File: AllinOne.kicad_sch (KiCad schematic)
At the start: 268 parts, among them SW0 SW_Push, SW1 SW_Push, SW10 SW_Push, SW100 SW_Push, SW101 SW_Push, SW102 SW_Push, SW103 SW_Push, SW104 SW_Push, SW105 SW_Push, SW106 SW_Push, SW107 SW_Push, SW108 SW_Push, SW109 SW_Push, SW11 SW_Push, SW110 SW_Push, SW111 SW_Push, SW114 SW_Push, SW116 SW_Push, SW117 SW_Push, SW118 SW_Push, SW119 SW_Push, SW12 SW_Push, SW120 SW_Push, SW121 SW_Push, SW122 SW_Push, SW126 SW_Push, SW13 SW_Push, SW130 SW_Push, SW131 SW_Push, SW132 SW_Push, SW133 SW_Push, SW134 SW_Push, SW135 SW_Push, SW136 SW_Push, SW137 SW_Push, SW138 SW_Push, SW139 SW_Push, SW14 SW_Push, SW15 SW_Push, SW16 SW_Push, SW18 SW_Push, SW19 SW_Push, SW2 SW_Push, SW20 SW_Push, SW21 SW_Push, SW22 SW_Push, SW23 SW_Push, SW24 SW_Push, SW25 SW_Push, SW26 SW_Push, SW27 SW_Push, SW28 SW_Push, SW29 SW_Push, SW3 SW_Push, SW30 SW_Push, SW31 SW_Push, SW32 SW_Push, SW33 SW_Push, SW34 SW_Push, SW35 SW_Push, SW36 SW_Push, SW37 SW_Push, SW38 SW_Push, SW39 SW_Push, SW4 SW_Push, SW40 SW_Push, SW41 SW_Push, SW42 SW_Push, SW43 SW_Push, SW44 SW_Push, SW45 SW_Push, SW46 SW_Push, SW47 SW_Push, SW48 SW_Push, SW49 SW_Push, SW5 SW_Push, SW50 SW_Push, SW51 SW_Push, SW52 SW_Push, SW53 SW_Push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

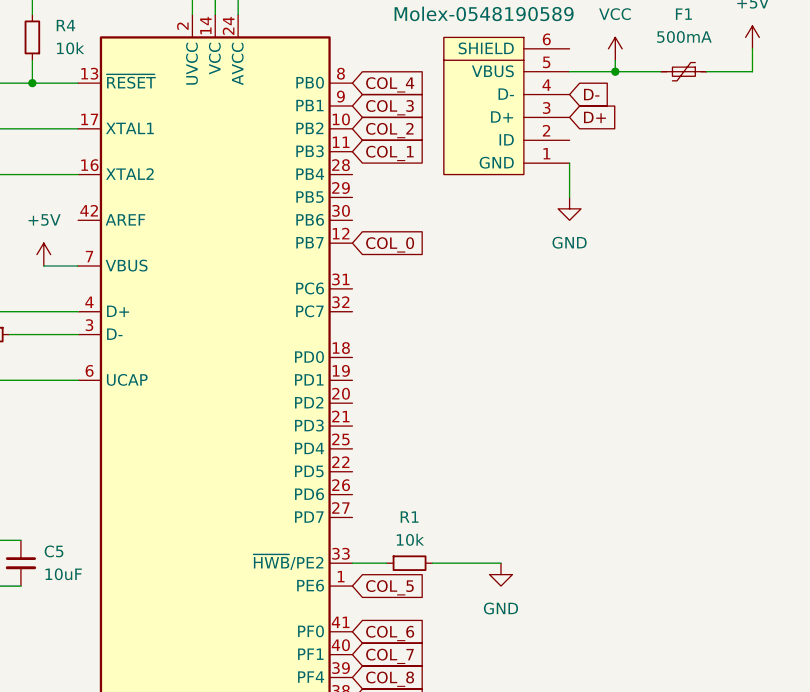
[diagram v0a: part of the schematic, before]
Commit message: All Done for now
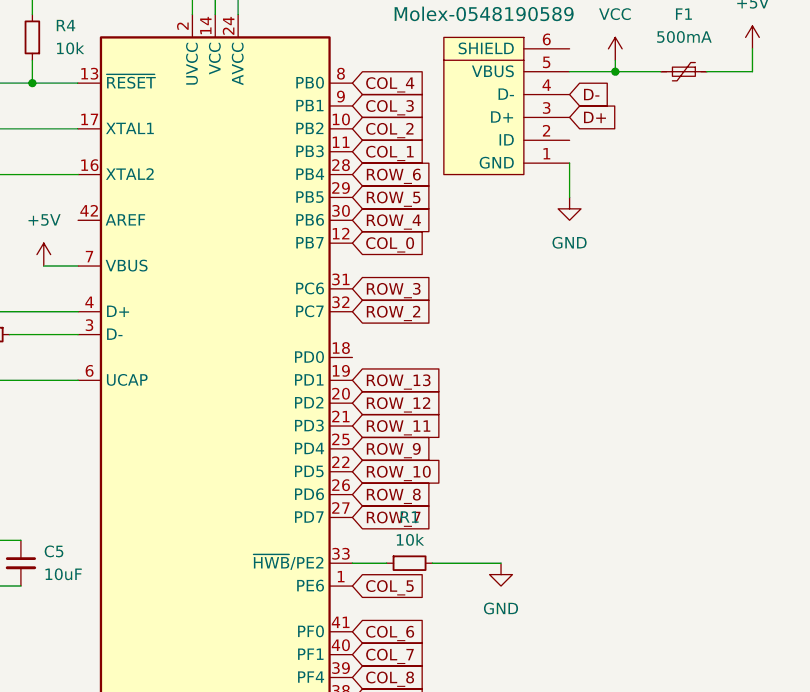
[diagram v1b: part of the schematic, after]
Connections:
- net ROW_10: now also U1.22 (PD5)
- net ROW_11: now also U1.21 (PD3)
- net ROW_12: now also U1.20 (PD2)
- net ROW_13: now also U1.19 (PD1)
- net ROW_2: now also U1.32 (PC7)
- net ROW_3: now also U1.31 (PC6)
- net ROW_4: now also U1.30 (PB6)
- net ROW_5: now also U1.29 (PB5)
- net ROW_6: now also U1.28 (PB4)
- net ROW_7: now also U1.27 (PD7)
- net ROW_8: now also U1.26 (PD6)
- net ROW_9: now also U1.25 (PD4)
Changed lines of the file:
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@@
     (stroke (width 0) (type default))
   )
+  (global_label "ROW_5" (shape input) (at 87.63 191.77 0) (fields_autoplaced)
+    (effects (font (size 1.27 1.27)) (justify left))
+    (property "Intersheetrefs" "${INTERSHEET_REFS}" (at 96.7648 191.77 0)
+      (effects (font (size 1.27 1.27)) (justify left) hide)
+    )
+  )
   (global_label "COL_6" (shape input) (at 289.56 27.94 90) (fields_autoplaced)
     (effects (font (size 1.27 1.27)) (justify left))
@@
     )
   )
+  (global_label "ROW_6" (shape input) (at 87.63 189.23 0) (fields_autoplaced)
+    (effects (font (size 1.27 1.27)) (justify left))
+    (property "Intersheetrefs" "${INTERSHEET_REFS}" (at 96.7648 189.23 0)
+      (effects (font (size 1.27 1.27)) (justify left) hide)
+    )
+  )
+  (global_label "ROW_10" (shape input) (at 87.63 222.25 0) (fields_autoplaced)
+    (effects (font (size 1.27 1.27)) (justify left))
+    (property "Intersheetrefs" "${INTERSHEET_REFS}" (at 97.9743 222.25 0)
+      (effects (font (size 1.27 1.27)) (justify left) hide)
+    )
+  )
   (global_label "ROW_7" (shape input) (at 30.48 109.22 180) (fields_autoplaced)
     (effects (font (size 1.27 1.27)) (justify right))
@@
     )
   )
+  (global_label "ROW_2" (shape input) (at 87.63 204.47 0) (fields_autoplaced)
+    (effects (font (size 1.27 1.27)) (justify left))
+    (property "Intersheetrefs" "${INTERSHEET_REFS}" (at 96.7648 204.47 0)
+      (effects (font (size 1.27 1.27)) (justify left) hide)
+    )
+  )
   (global_label "COL_0" (shape input) (at 76.2 27.94 90) (fields_autoplaced)
     (effects (font (size 1.27 1.27)) (justify left))
@@
     )
   )
+  (global_label "ROW_7" (shape input) (at 87.63 227.33 0) (fields_autoplaced)
+    (effects (font (size 1.27 1.27)) (justify left))
+    (property "Intersheetrefs" "${INTERSHEET_REFS}" (at 96.7648 227.33 0)
+      (effects (font (size 1.27 1.27)) (justify left) hide)
+    )
+  )
   (global_label "COL_7" (shape input) (at 87.63 242.57 0) (fields_autoplaced)
     (effects (font (size 1.27 1.27)) (justify left))
@@
     )
   )
+  (global_label "ROW_8" (shape input) (at 87.63 224.79 0) (fields_autoplaced)
+    (effects (font (size 1.27 1.27)) (justify left))
+    (property "Intersheetrefs" "${INTERSHEET_REFS}" (at 96.7648 224.79 0)
+      (effects (font (size 1.27 1.27)) (justify left) hide)
+    )
+  )
   (global_label "ROW_0" (shape input) (at 87.63 250.19 0) (fields_autoplaced)
     (effects (font (size 1.27 1.27)) (justify left))
@@
     )
   )
+  (global_label "ROW_12" (shape input) (at 87.63 214.63 0) (fields_autoplaced)
+    (effects (font (size 1.27 1.27)) (justify left))
+    (property "Intersheetrefs" "${INTERSHEET_REFS}" (at 97.9743 214.63 0)
+      (effects (font (size 1.27 1.27)) (justify left) hide)
+    )
+  )
   (global_label "COL_3" (shape input) (at 182.88 27.94 90) (fields_autoplaced)
     (effects (font (size 1.27 1.27)) (justify left))
@@
     )
   )
+  (global_label "ROW_3" (shape input) (at 87.63 201.93 0) (fields_autoplaced)
+    (effects (font (size 1.27 1.27)) (justify left))
+    (property "Intersheetrefs" "${INTERSHEET_REFS}" (at 96.7648 201.93 0)
+      (effects (font (size 1.27 1.27)) (justify left) hide)
+    )
+  )
+  (global_label "ROW_11" (shape input) (at 87.63 217.17 0) (fields_autoplaced)
+    (effects (font (size 1.27 1.27)) (justify left))
+    (property "Intersheetrefs" "${INTERSHEET_REFS}" (at 97.9743 217.17 0)
+      (effects (font (size 1.27 1.27)) (justify left) hide)
+    )
+  )
   (global_label "ROW_11" (shape input) (at 30.48 139.7 180) (fields_autoplaced)
     (effects (font (size 1.27 1.27)) (justify right))
@@
     )
   )
+  (global_label "ROW_9" (shape input) (at 87.63 219.71 0) (fields_autoplaced)
+    (effects (font (size 1.27 1.27)) (justify left))
+    (property "Intersheetrefs" "${INTERSHEET_REFS}" (at 96.7648 219.71 0)
+      (effects (font (size 1.27 1.27)) (justify left) hide)
+    )
+  )
+  (global_label "ROW_13" (shape input) (at 87.63 212.09 0) (fields_autoplaced)
+    (effects (font (size 1.27 1.27)) (justify left))
+    (property "Intersheetrefs" "${INTERSHEET_REFS}" (at 97.9743 212.09 0)
+      (effects (font (size 1.27 1.27)) (justify left) hide)
+    )
+  )
   (global_label "COL_5" (shape input) (at 254 27.94 90) (fields_autoplaced)
     (effects (font (size 1.27 1.27)) (justify left))
@@
       (effects (font (size 1.27 1.27)) (justify left) hide)
     )
+  )
+  (global_label "ROW_4" (shape input) (at 87.63 194.31 0) (fields_autoplaced)
+    (effects (font (size 1.27 1.27)) (justify left))
+    (property "Intersheetrefs" "${INTERSHEET_REFS}" (at 96.7648 194.31 0)
+      (effects (font (size 1.27 1.27)) (justify left) hide)
+    )
